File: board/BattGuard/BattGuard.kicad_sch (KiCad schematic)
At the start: 7 parts, among them J1 OQ0271510000G, U1 BQ25756ERRVR, U2 ESP32-S3-WROOM-1, U3 LM317_TO3

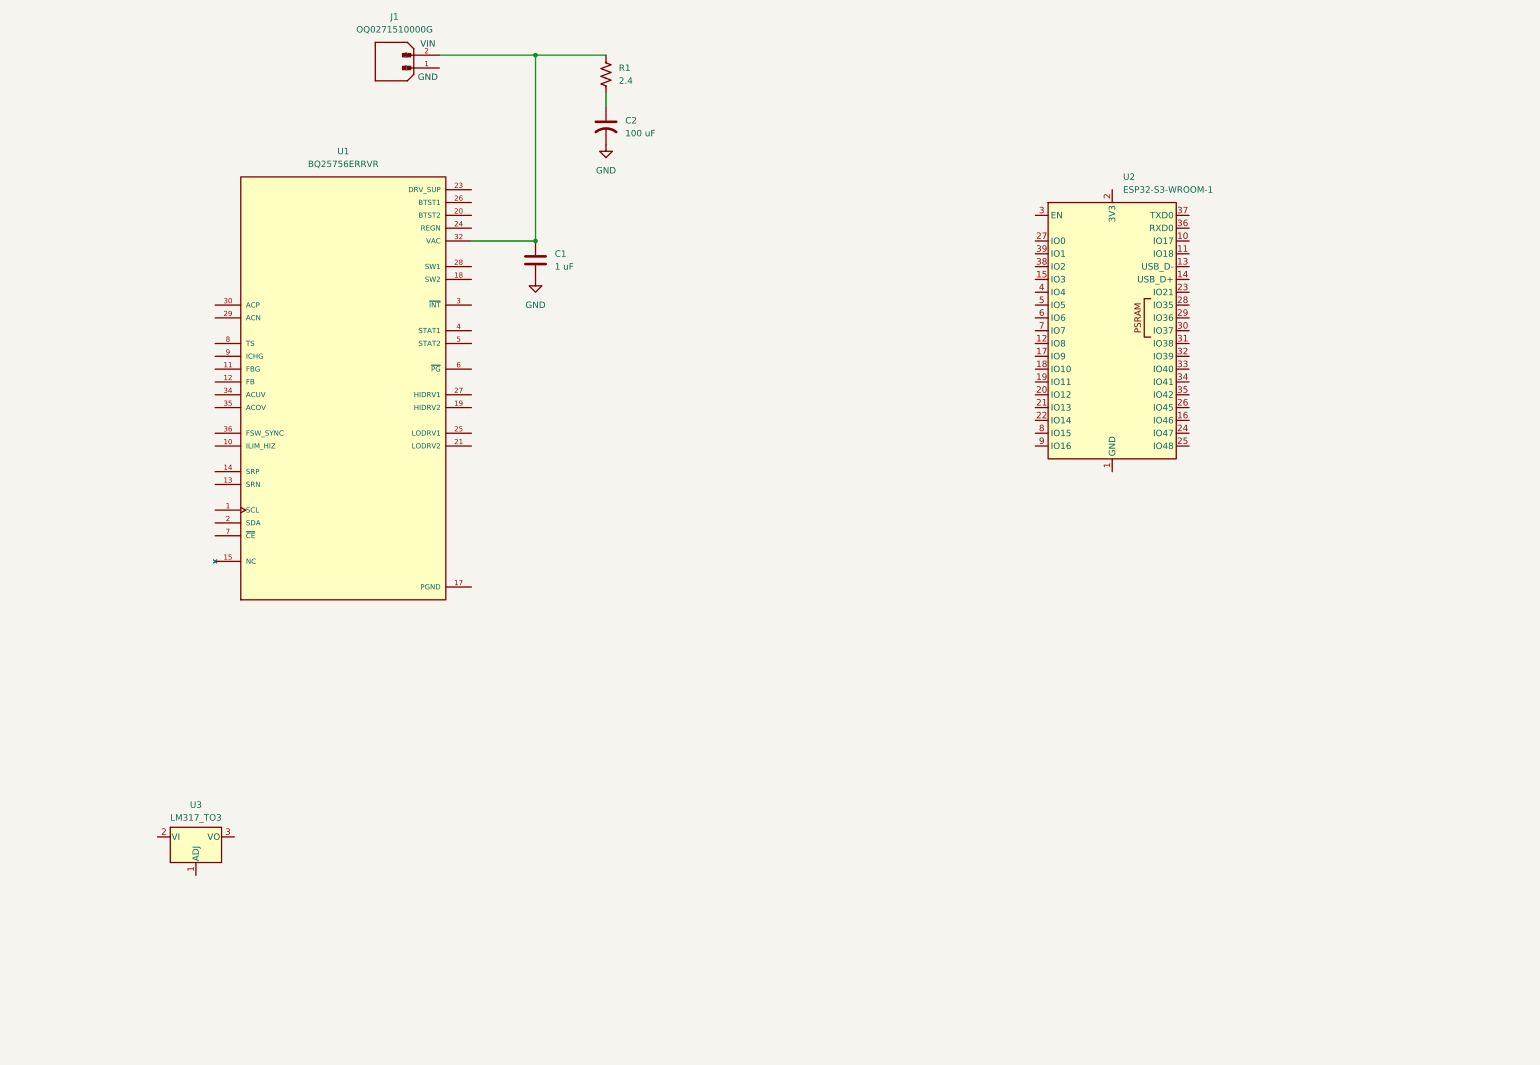
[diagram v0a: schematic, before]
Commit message: 10.16.2026
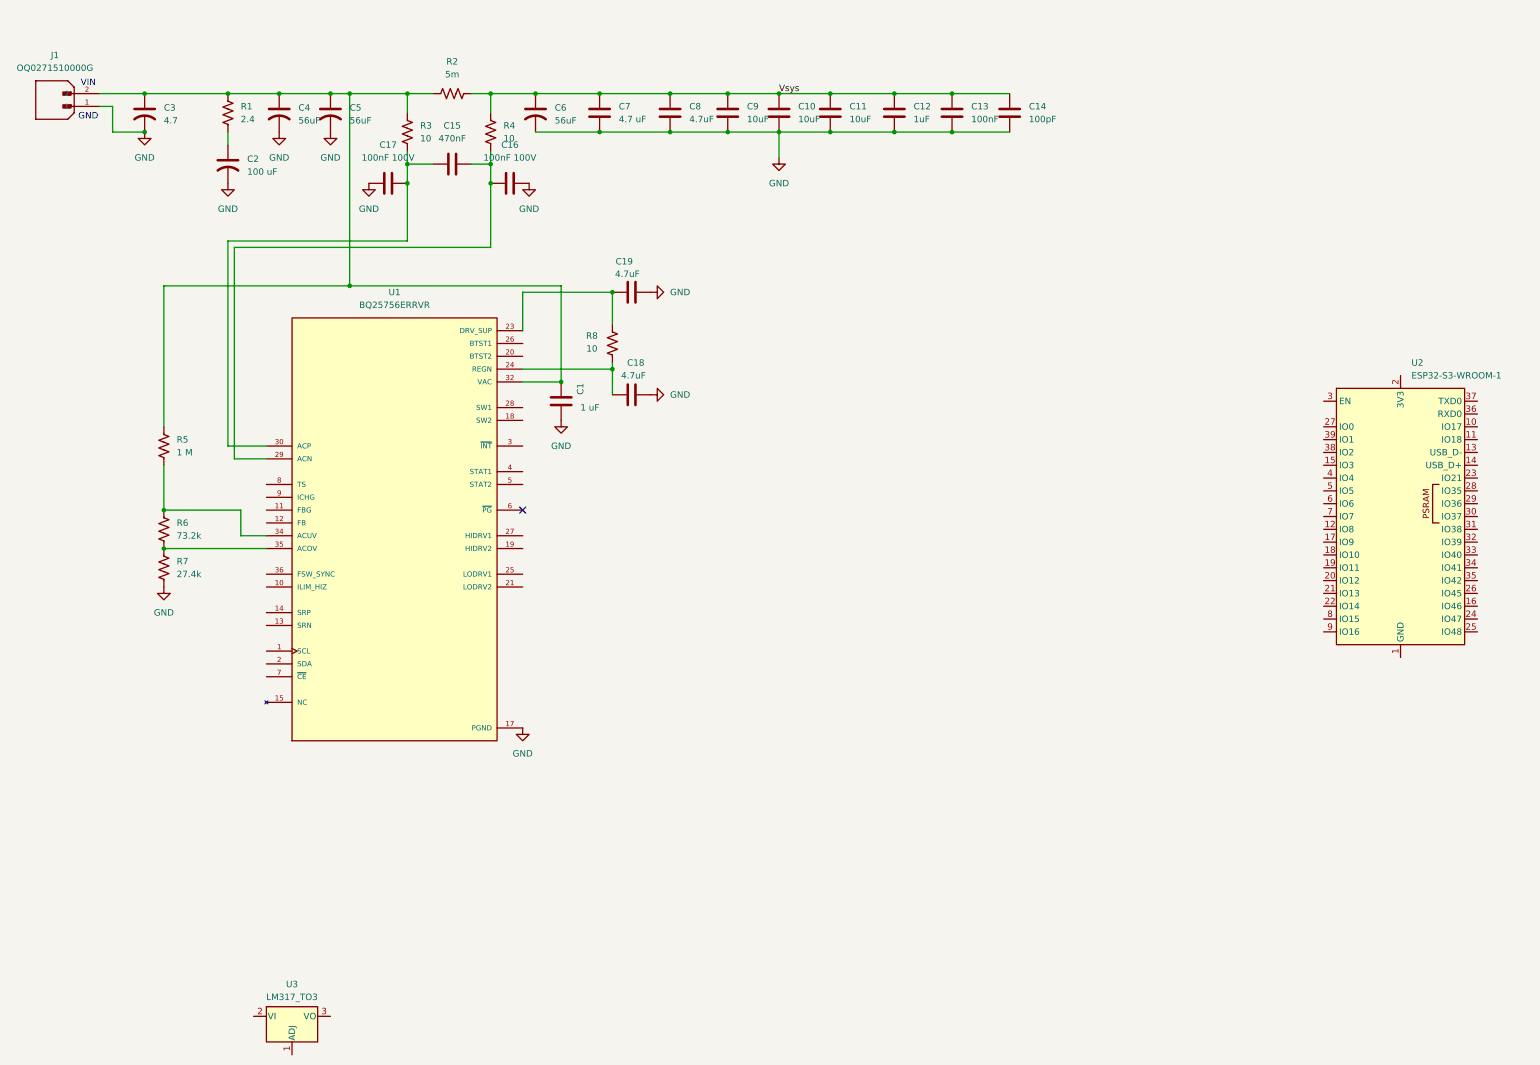
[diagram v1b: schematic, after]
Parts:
- added C10, C11, C9: 10uF, symbol Device:C
- added C12: 1uF, symbol Device:C
- added C13: 100nF, symbol Device:C
- added C14: 100pF, symbol Device:C
- added C15: 470nF, symbol Device:C
- added C16, C17: 100nF 100V, symbol Device:C
- added C18, C19, C8: 4.7uF, symbol Device:C
- added C3: 4.7, symbol Device:C_US
- added C4, C5, C6: 56uF, symbol Device:C_US
- added C7: 4.7 uF, symbol Device:C
- added R2: 5m, symbol Device:R_US
- added R3, R4, R8: 10, symbol Device:R_US
- added R5: 1 M, symbol Device:R_US
- added R6: 73.2k, symbol Device:R_US
- added R7: 27.4k, symbol Device:R_US
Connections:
- net PGND is gone; now on net GND: U1.17 (PGND), U1.22 (PGND), U1.37 (PGND)
- net GND: now also J1.1, C10.2, C11.2, C12.2, C13.2, C14.2, C16.2, C17.1, C18.2, C19.2, C3.2, C4.2, C5.2, C6.2, C7.2, C8.2, C9.2, R7.2
- net VAC: now also C3.1, C4.1, C5.1, R2.1, R3.1, R5.1
- net at U1.23 (DRV_SUP): now also C19.1, R8.2
- net at U1.24 (REGN): now also C18.1, R8.1
- net at U1.29 (ACN): now also C15.2, C16.1, R4.2
- net at U1.30 (ACP): now also C15.1, C17.2, R3.2
- net at U1.34 (ACUV): now also R5.2, R6.1
- net at U1.35 (ACOV): now also R6.2, R7.1
- new net Vsys: C10.1, C11.1, C12.1, C13.1, C14.1, C6.1, C7.1, C8.1, C9.1, R2.2, R4.1
- no-connect marks 0 -> 1
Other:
- moved on the sheet: C1, C2, J1, R1, U1, U2, U3
